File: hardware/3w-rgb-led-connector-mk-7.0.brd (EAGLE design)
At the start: 52 x 39 mm, 8 parts, among them U1 SHEELD, U2 ADAFRUIT_9DOF_BREAKOUTHOLEY, U3 ADAFRUIT_BLE_UARTHOLEY-MOLEY

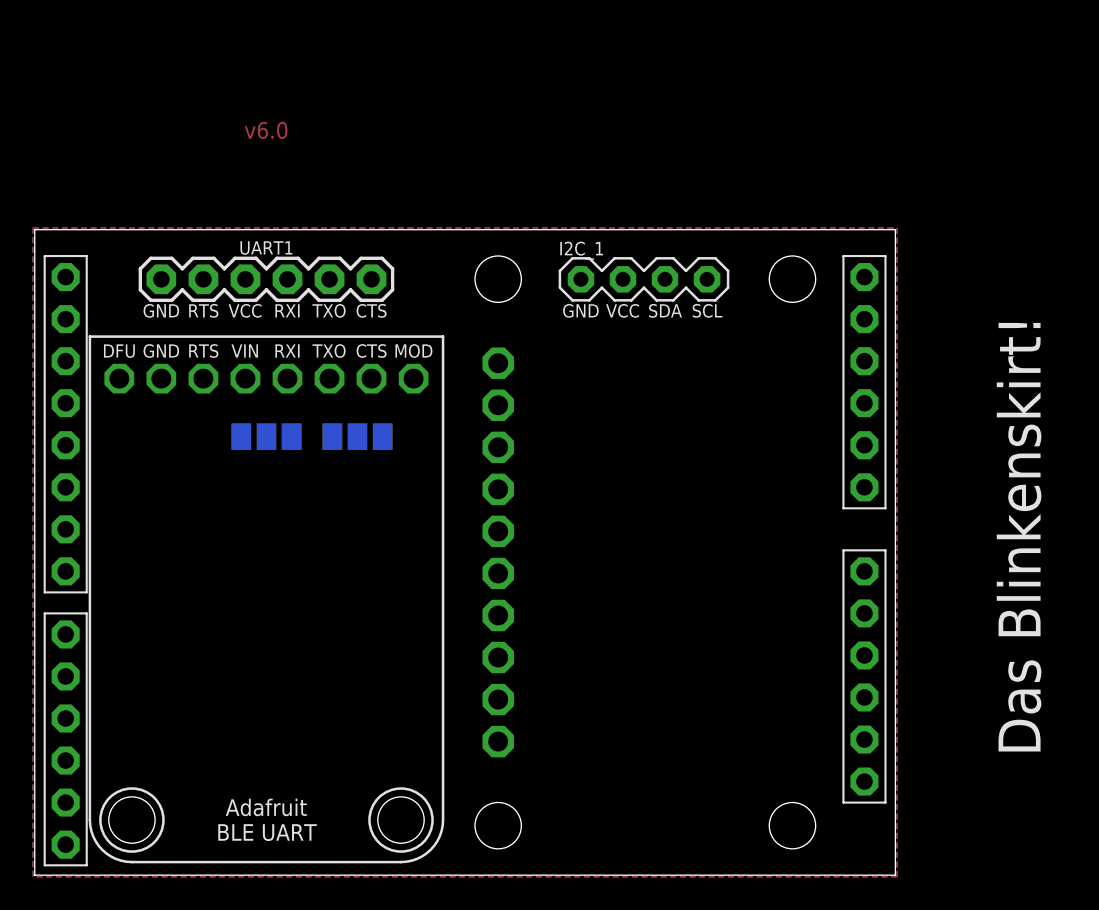
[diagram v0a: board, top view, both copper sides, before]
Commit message: dotstarstick
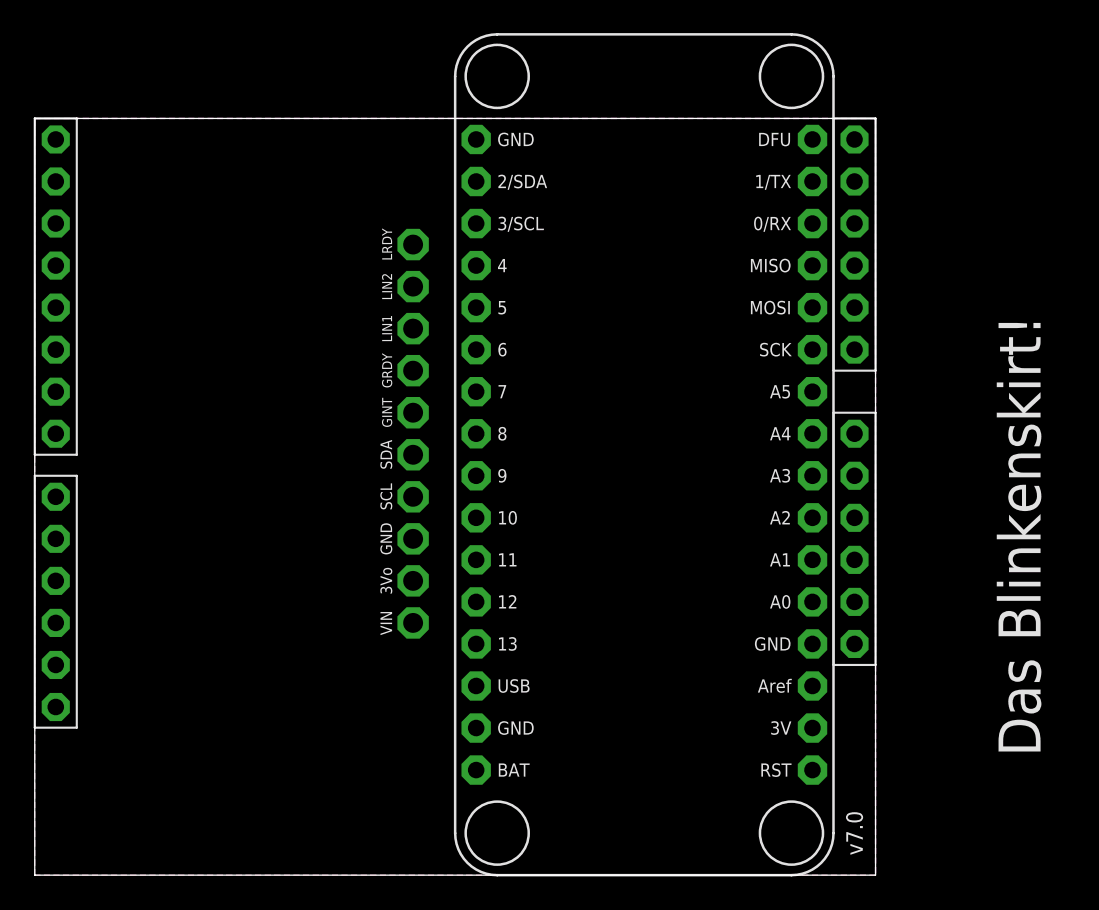
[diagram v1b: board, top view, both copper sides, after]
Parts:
- removed I2C_1: M04-I2CPTH-0.1IN, A_butts:1X04-PTH-VERT-I2C
- removed RXI, TXO: (no value), A_butts:PAD-JUMPER-3-NO_YES_SILK_FULL_BOX
- removed UART1: M06-UARTPTH-0.1IN, A_butts:1X06_PTH_UART
- FRAME1: value (none) -> FRAME-LETTERNO_PACKAGE
- U2: value ADAFRUIT_9DOF_BREAKOUTHOLEY -> ADAFRUIT_BLUEFRUIT_LE_MICRO; device A_butts:ADAFRUIT_9DOF_BREAKOUT_HOLEY -> A_butts:ADAFRUIT_BLUEFRUIT_LE_MICRO
- U3: value ADAFRUIT_BLE_UARTHOLEY-MOLEY -> ADAFRUIT_9DOF_BREAKOUT; device A_butts:ADAFRUIT_BLE_UART_HOLEY -> A_butts:ADAFRUIT_9DOF_BREAKOUT
- moved U2 10.6 mm to (36.8, 25.4), flipped to the top
- moved U3 9.47 mm to (22.9, 26.7), turned to 90 degrees
- moved U1 8.34 mm to (1.27, 44.5)
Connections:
- removed net RX: TXO.1, U1.RX
- removed net RXI: RXI.2, U3.RXI, UART1.RXI
- removed net TX: RXI.1, U1.TX
- removed net TXO: TXO.2, U3.TXO, UART1.TXO
- new net 3.3V: U1.3.3V, U2.3V3
- net 5V: now also U2.BAT; no longer I2C_1.VCC, U2.VIN, UART1.VCC
- net D2: no longer U3.CTS, UART1.CTS
- net D4: no longer U3.DFU
- net D5: no longer U3.RTS, UART1.RTS
- net D6: no longer RXI.3
- net D7: no longer TXO.3
- net D8: no longer U3.MOD
- net GND: now also U2.GND@1, U2.GND@2, U2.GND@3; no longer I2C_1.GND, U2.GND, UART1.GND
- net SCL: now also U2.3/SCL, U3.SCL; no longer I2C_1.SDA, U2.SCL
- net SDA: now also U2.2/SDA, U3.SDA; no longer I2C_1.SCL, U2.SDA
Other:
- board size 52 x 39 mm -> 50.8 x 45.7 mm
- board text removed: "D0"
- board text removed: "D1"
- board text removed: "D6"
- board text removed: "D7"
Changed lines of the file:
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@@
 <setting verticaltext="up"/>
 </settings>
-<grid distance="0.5" unitdist="mm" unit="mm" style="lines" multiple="2" display="yes" altdistance="1" altunitdist="mil" altunit="mil"/>
+<grid distance="25" unitdist="mil" unit="mil" style="lines" multiple="2" display="yes" altdistance="1" altunitdist="mil" altunit="mil"/>
 <layers>
 <layer number="1" name="Top" color="4" fill="1" visible="yes" active="yes"/>
@@
 <board>
 <plain>
-<wire x1="0" y1="0" x2="52" y2="0" width="0" layer="20"/>
-<wire x1="52" y1="0" x2="52" y2="39" width="0" layer="20"/>
-<wire x1="52" y1="39" x2="0" y2="39" width="0" layer="20"/>
-<wire x1="0" y1="39" x2="0" y2="0" width="0" layer="20"/>
+<wire x1="0" y1="0" x2="50.8" y2="0" width="0" layer="20"/>
+<wire x1="50.8" y1="0" x2="50.8" y2="45.72" width="0" layer="20"/>
+<wire x1="50.8" y1="45.72" x2="0" y2="45.72" width="0" layer="20"/>
+<wire x1="0" y1="45.72" x2="0" y2="0" width="0" layer="20"/>
 <text x="59.5" y="20.5" size="2.54" layer="21" font="vector" ratio="12" rot="R90" align="center">Das Blinkenskirt!</text>
-<text x="15.81" y="28.04" size="0.7" layer="22" font="vector" ratio="12" rot="MR0" align="bottom-center">D6</text>
-<text x="21.19" y="28" size="0.7" layer="22" font="vector" ratio="12" rot="MR0" align="bottom-center">D7</text>
-<text x="17.61" y="28" size="0.7" layer="22" font="vector" ratio="12" rot="MR0" align="bottom-center">D0</text>
-<text x="12.23" y="28" size="0.7" layer="22" font="vector" ratio="12" rot="MR0" align="bottom-center">D1</text>
-<text x="14" y="45" size="1" layer="1" font="vector" ratio="12" align="center">&gt;VERSION</text>
-<text x="14" y="45" size="1" layer="21" font="vector" ratio="12" align="center">&gt;VERSION</text>
+<text x="49.53" y="2.54" size="1" layer="21" font="vector" ratio="16" rot="R90" align="center">&gt;VERSION</text>
+<text x="49.53" y="2.54" size="1" layer="1" font="vector" ratio="16" rot="R90" align="center">&gt;VERSION</text>
 </plain>
 <attributes>
-<attribute name="VERSION" value="v6.0"/>
+<attribute name="VERSION" value="v7.0"/>
 </attributes>
 <variantdefs>
@@
 </autorouter>
 <elements>
-<element name="FRAME1" library="A_butts" package="DUMMY" value="" x="0" y="0">
-<attribute name="VERSION" value="v6.0" x="0" y="0" size="0.5" layer="27" ratio="12" display="off"/>
+<element name="FRAME1" library="A_butts" package="DUMMY" value="FRAME-LETTERNO_PACKAGE" x="0" y="0">
+<attribute name="VERSION" value="v7.0" x="0" y="0" size="0.5" layer="27" ratio="12" display="off"/>
 <attribute name="DESIGNER" value="sean@yak.net" x="0" y="0" size="0.5" layer="27" ratio="12" display="off"/>
 </element>
-<element name="U1" library="A_butts" package="ARDUINO_SHIELD_NOOUTLINE_INSIDE_SMALLER" value="SHEELD" x="1.87" y="36.135"/>
-<element name="U2" library="A_butts" package="ADAFRUIT_9DOF_BREAKOUT_HOLEY" value="ADAFRUIT_9DOF_BREAKOUTHOLEY" x="28" y="19.5" rot="MR90"/>
-<element name="U3" library="A_butts" package="ADAFRUIT_BLE_UART_HOLEY" value="ADAFRUIT_BLE_UARTHOLEY-MOLEY" x="14" y="30" rot="R180"/>
-<element name="I2C_1" library="A_butts" package="1X04-PTH-VERT-I2C" value="M04-I2CPTH-0.1IN" x="33" y="36"/>
-<element name="UART1" library="A_butts" package="1X06_PTH_UART" value="M06-UARTPTH-0.1IN" x="7.65" y="36"/>
-<element name="TXO" library="A_butts" package="PAD-JUMPER-3-NO_YES_SILK_FULL_BOX" value="" x="19.5" y="26.5" rot="MR180"/>
-<element name="RXI" library="A_butts" package="PAD-JUMPER-3-NO_YES_SILK_FULL_BOX" value="" x="14" y="26.5" rot="MR180"/>
+<element name="U1" library="A_butts" package="ARDUINO_SHIELD_NOOUTLINE_INSIDE_SMALLER" value="SHEELD" x="1.27" y="44.45"/>
+<element name="U3" library="A_butts" package="ADAFRUIT_9DOF_BREAKOUT" value="ADAFRUIT_9DOF_BREAKOUT" x="22.86" y="26.67" rot="R90"/>
+<element name="U2" library="A_butts" package="ADAFRUIT_BLUEFRUIT_LE_MICRO" value="ADAFRUIT_BLUEFRUIT_LE_MICRO" x="36.83" y="25.4" rot="R90"/>
 </elements>
 <signals>
 <signal name="SDA">
 <contactref element="U1" pad="A4"/>
-<contactref element="U2" pad="SDA"/>
-<contactref element="I2C_1" pad="SCL"/>
-<wire x1="40.62" y1="36" x2="50.13" y2="33.595" width="0" layer="19" extent="1-1"/>
-<wire x1="28" y1="18.23" x2="40.62" y2="36" width="0" layer="19" extent="1-1"/>
+<contactref element="U3" pad="SDA"/>
+<contactref element="U2" pad="2/SDA"/>
+<wire x1="26.67" y1="41.91" x2="49.53" y2="41.91" width="0" layer="19" extent="1-1"/>
+<wire x1="22.86" y1="25.4" x2="26.67" y2="41.91" width="0" layer="19" extent="1-1"/>
 </signal>
 <signal name="SCL">
 <contactref element="U1" pad="A5"/>
-<contactref element="U2" pad="SCL"/>
-<contactref element="I2C_1" pad="SDA"/>
-<wire x1="38.08" y1="36" x2="50.13" y2="36.135" width="0" layer="19" extent="1-1"/>
-<wire x1="28" y1="15.69" x2="38.08" y2="36" width="0" layer="19" extent="1-1"/>
+<contactref element="U3" pad="SCL"/>
+<contactref element="U2" pad="3/SCL"/>
+<wire x1="26.67" y1="39.37" x2="49.53" y2="44.45" width="0" layer="19" extent="1-1"/>
+<wire x1="22.86" y1="22.86" x2="26.67" y2="39.37" width="0" layer="19" extent="1-1"/>
 </signal>
 <signal name="GND">
@@
 <contactref element="U1" pad="GND@1"/>
 <polygon width="0.1524" layer="1" isolate="0.1524">
-<vertex x="-0.1" y="39.1"/>
-<vertex x="52.1" y="39.1"/>
-<vertex x="52.1" y="-0.1"/>
-<vertex x="-0.1" y="-0.1"/>
+<vertex x="0" y="45.72"/>
+<vertex x="50.8" y="45.72"/>
+<vertex x="50.8" y="0"/>
+<vertex x="0" y="0"/>
 </polygon>
 <polygon width="0.1524" layer="16" isolate="0.1524">
-<vertex x="-0.1" y="-0.1"/>
-<vertex x="-0.1" y="39.1"/>
-<vertex x="52.1" y="39.1"/>
-<vertex x="52.1" y="-0.1"/>
+<vertex x="0" y="0"/>
+<vertex x="0" y="45.72"/>
+<vertex x="50.8" y="45.72"/>
+<vertex x="50.8" y="0"/>
 </polygon>
-<contactref element="U2" pad="GND"/>
 <contactref element="U3" pad="GND"/>
-<contactref element="UART1" pad="GND"/>
-<contactref element="I2C_1" pad="GND"/>
+<contactref element="U2" pad="GND@1"/>
+<contactref element="U2" pad="GND@2"/>
+<contactref element="U2" pad="GND@3"/>
 </signal>
 <signal name="5V">
 <contactref element="U1" pad="5V"/>
-<contactref element="U2" pad="VIN"/>
 <contactref element="U3" pad="VIN"/>
-<contactref element="UART1" pad="VCC"/>
-<contactref element="I2C_1" pad="VCC"/>
-<wire x1="12.73" y1="36" x2="35.54" y2="36" width="0" layer="19" extent="1-1"/>
-<wire x1="12.73" y1="30" x2="12.73" y2="36" width="0" layer="19" extent="1-1"/>
-<wire x1="28" y1="8.07" x2="12.73" y2="30" width="0" layer="19" extent="1-1"/>
-<wire x1="50.13" y1="10.735" x2="28" y2="8.07" width="0" layer="19" extent="1-1"/>
-</signal>
-<signal name="TXO">
-<contactref element="U3" pad="TXO"/>
-<contactref element="UART1" pad="TXO"/>
-<contactref element="TXO" pad="2"/>
-<wire x1="17.81" y1="30" x2="17.81" y2="36" width="0" layer="19" extent="1-1"/>
-<wire x1="19.5" y1="26.5" x2="17.81" y2="30" width="0" layer="19" extent="16-16"/>
-</signal>
-<signal name="RXI">
-<contactref element="U3" pad="RXI"/>
-<contactref element="UART1" pad="RXI"/>
-<contactref element="RXI" pad="2"/>
-<wire x1="15.27" y1="30" x2="15.27" y2="36" width="0" layer="19" extent="1-1"/>
-<wire x1="14" y1="26.5" x2="15.27" y2="30" width="0" layer="19" extent="16-16"/>
+<contactref element="U2" pad="BAT"/>
+<wire x1="26.67" y1="6.35" x2="49.53" y2="19.05" width="0" layer="19" extent="1-1"/>
+<wire x1="22.86" y1="15.24" x2="26.67" y2="6.35" width="0" layer="19" extent="1-1"/>
 </signal>
 <signal name="D2">
 <contactref element="U1" pad="D2"/>
-<contactref element="U3" pad="CTS"/>
-<contactref element="UART1" pad="CTS"/>
-<wire x1="20.35" y1="30" x2="20.35" y2="36" width="0" layer="19" extent="1-1"/>
-<wire x1="1.87" y1="31.055" x2="20.35" y2="30" width="0" layer="19" extent="1-1"/>
 </signal>
 <signal name="D8">
 <contactref element="U1" pad="D8"/>
-<contactref element="U3" pad="MOD"/>
-<wire x1="1.87" y1="14.545" x2="22.89" y2="30" width="0" layer="19" extent="1-1"/>
-</signal>
-<signal name="RX">
-<contactref element="U1" pad="RX"/>
-<contactref element="TXO" pad="1"/>
-<wire x1="1.87" y1="36.135" x2="17.976" y2="26.5" width="0" layer="19" extent="16-16"/>
-</signal>
-<signal name="TX">
-<contactref element="U1" pad="TX"/>
-<contactref element="RXI" pad="1"/>
-<wire x1="1.87" y1="33.595" x2="12.476" y2="26.5" width="0" layer="19" extent="16-16"/>
 </signal>
 <signal name="D7">
 <contactref element="U1" pad="D7"/>
-<contactref element="TXO" pad="3"/>
-<wire x1="1.87" y1="18.355" x2="21.024" y2="26.5" width="0" layer="19" extent="16-16"/>
 </signal>
 <signal name="D6">
 <contactref element="U1" pad="D6"/>
-<contactref element="RXI" pad="3"/>
-<wire x1="1.87" y1="20.895" x2="15.524" y2="26.5" width="0" layer="19" extent="16-16"/>
 </signal>
 <signal name="D5">
 <contactref element="U1" pad="D5"/>
-<contactref element="U3" pad="RTS"/>
-<contactref element="UART1" pad="RTS"/>
-<wire x1="10.19" y1="30" x2="10.19" y2="36" width="0" layer="19" extent="1-1"/>
-<wire x1="1.87" y1="23.435" x2="10.19" y2="30" width="0" layer="19" extent="1-1"/>
 </signal>
 <signal name="D4">
 <contactref element="U1" pad="D4"/>
-<contactref element="U3" pad="DFU"/>
-<wire x1="1.87" y1="25.975" x2="5.11" y2="30" width="0" layer="19" extent="1-1"/>
+</signal>
+<signal name="3.3V">
+<contactref element="U1" pad="3.3V"/>
+<contactref element="U2" pad="3V3"/>
+<wire x1="46.99" y1="8.89" x2="49.53" y2="16.51" width="0" layer="19" extent="1-1"/>
 </signal>
 </signals>
